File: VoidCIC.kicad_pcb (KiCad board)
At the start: 2 copper layers, 11.5 x 23 mm, 8 parts, among them U1 SN74LVC1GU04DBVR

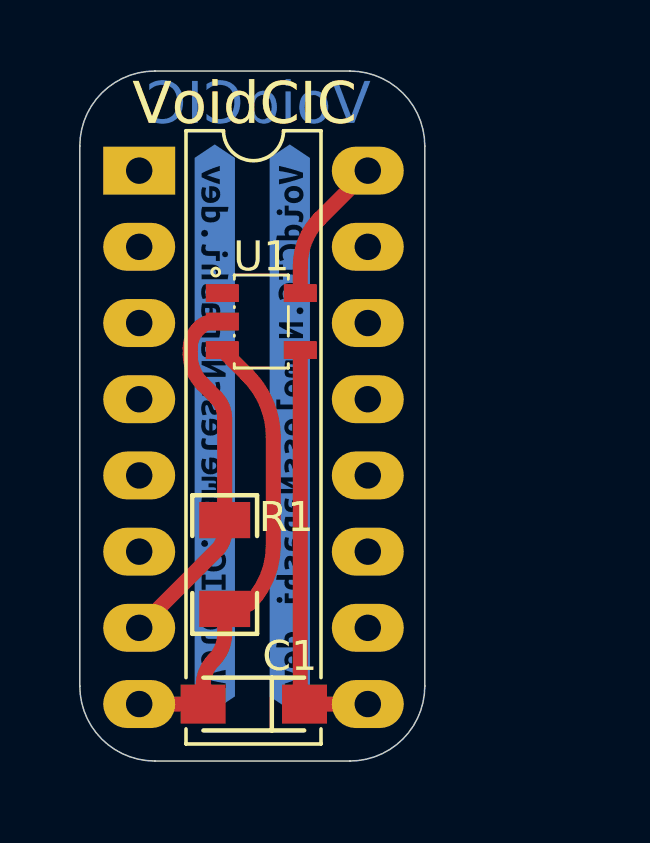
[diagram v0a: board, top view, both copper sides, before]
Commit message: update production after linting
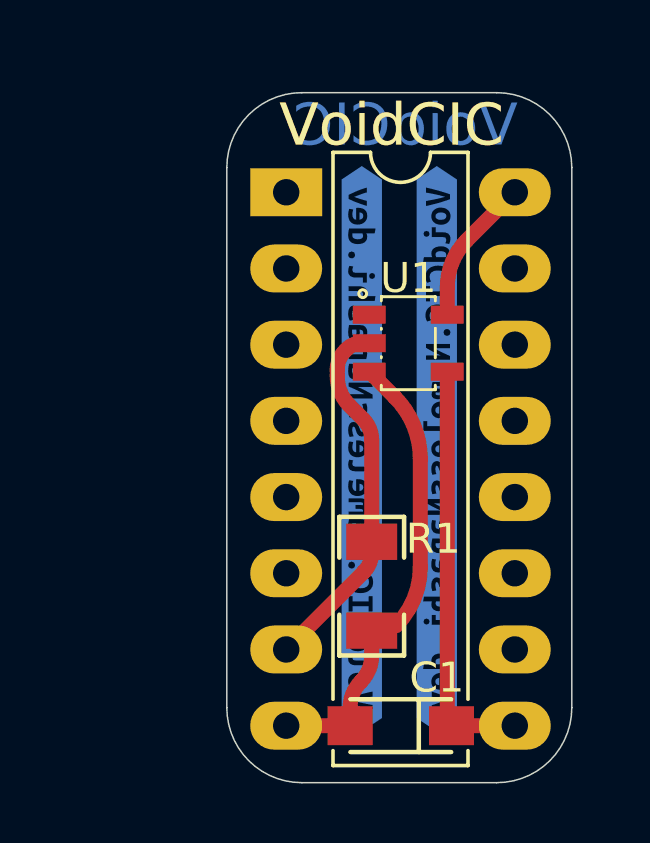
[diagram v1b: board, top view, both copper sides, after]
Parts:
- moved C1 4.95 mm to (155.8, 108.1)
- moved U1 4.95 mm to (156.1, 95.4)
- moved VoidCIC1 4.95 mm to (152.0, 90.3)
- moved R1 4.95 mm to (154.8, 103.5)
- moved kibuzzard-675A635B 4.95 mm to (157.0, 98.9)
- moved kibuzzard-675A635B 4.95 mm to (154.5, 98.9)
- moved kibuzzard-675A6399 4.95 mm to (157.0, 98.9)
- moved kibuzzard-675A6399 4.95 mm to (154.5, 98.9)
